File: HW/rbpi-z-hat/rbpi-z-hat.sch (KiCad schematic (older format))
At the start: 5 parts, among them Q1 DMG2302U

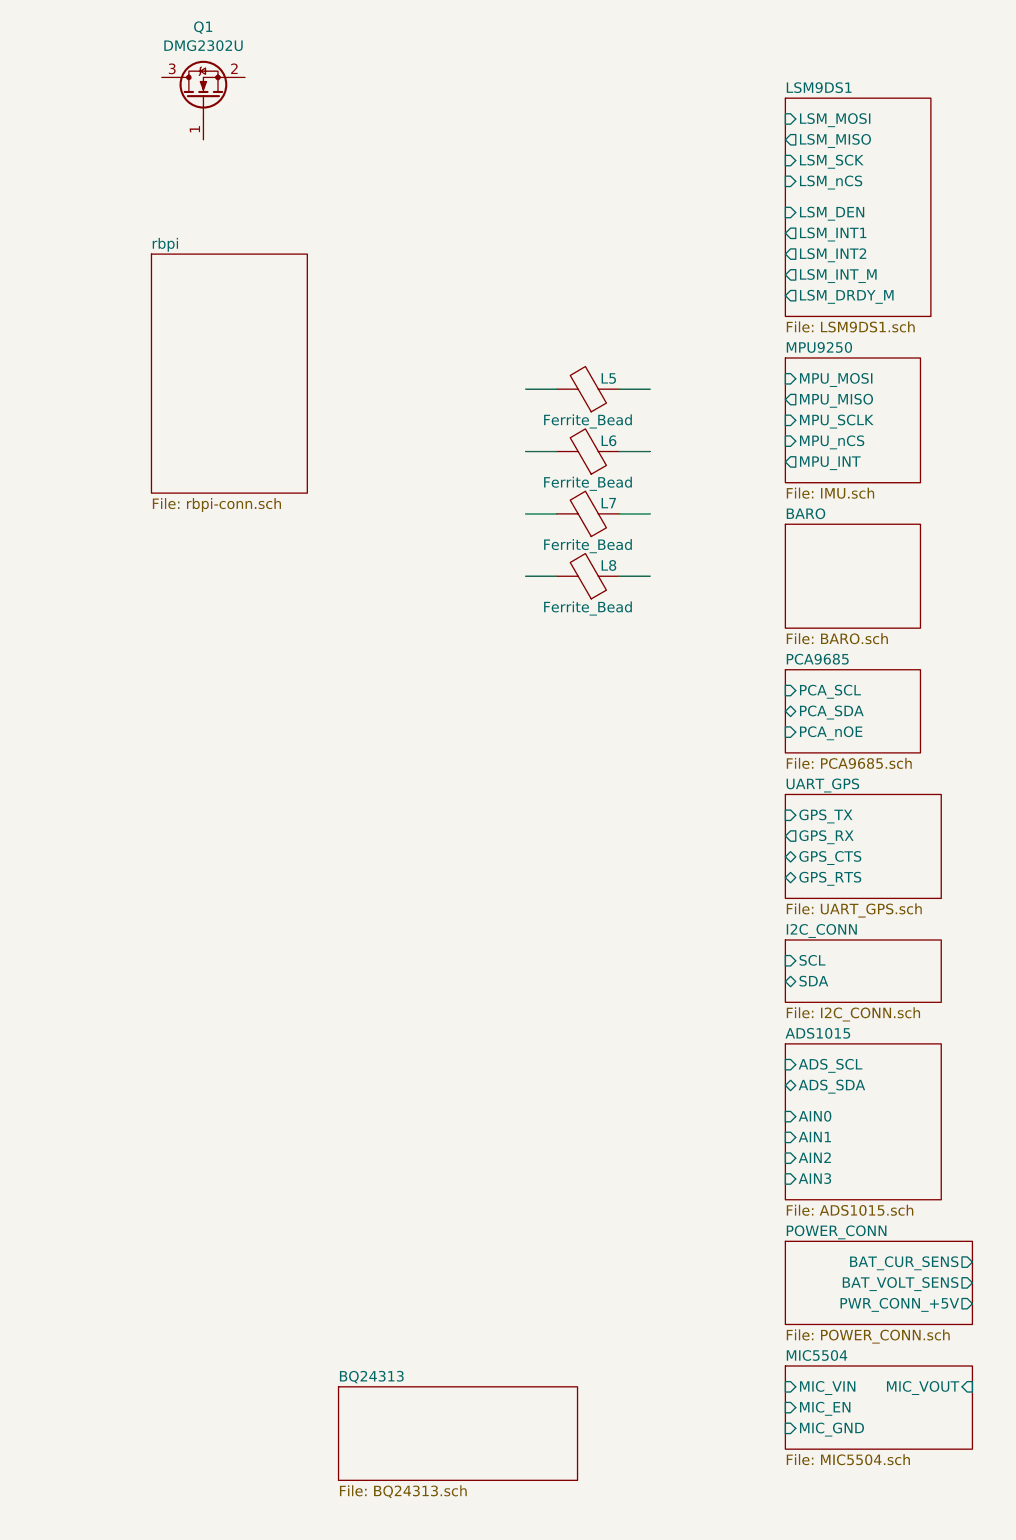
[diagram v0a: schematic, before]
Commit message: Commit...
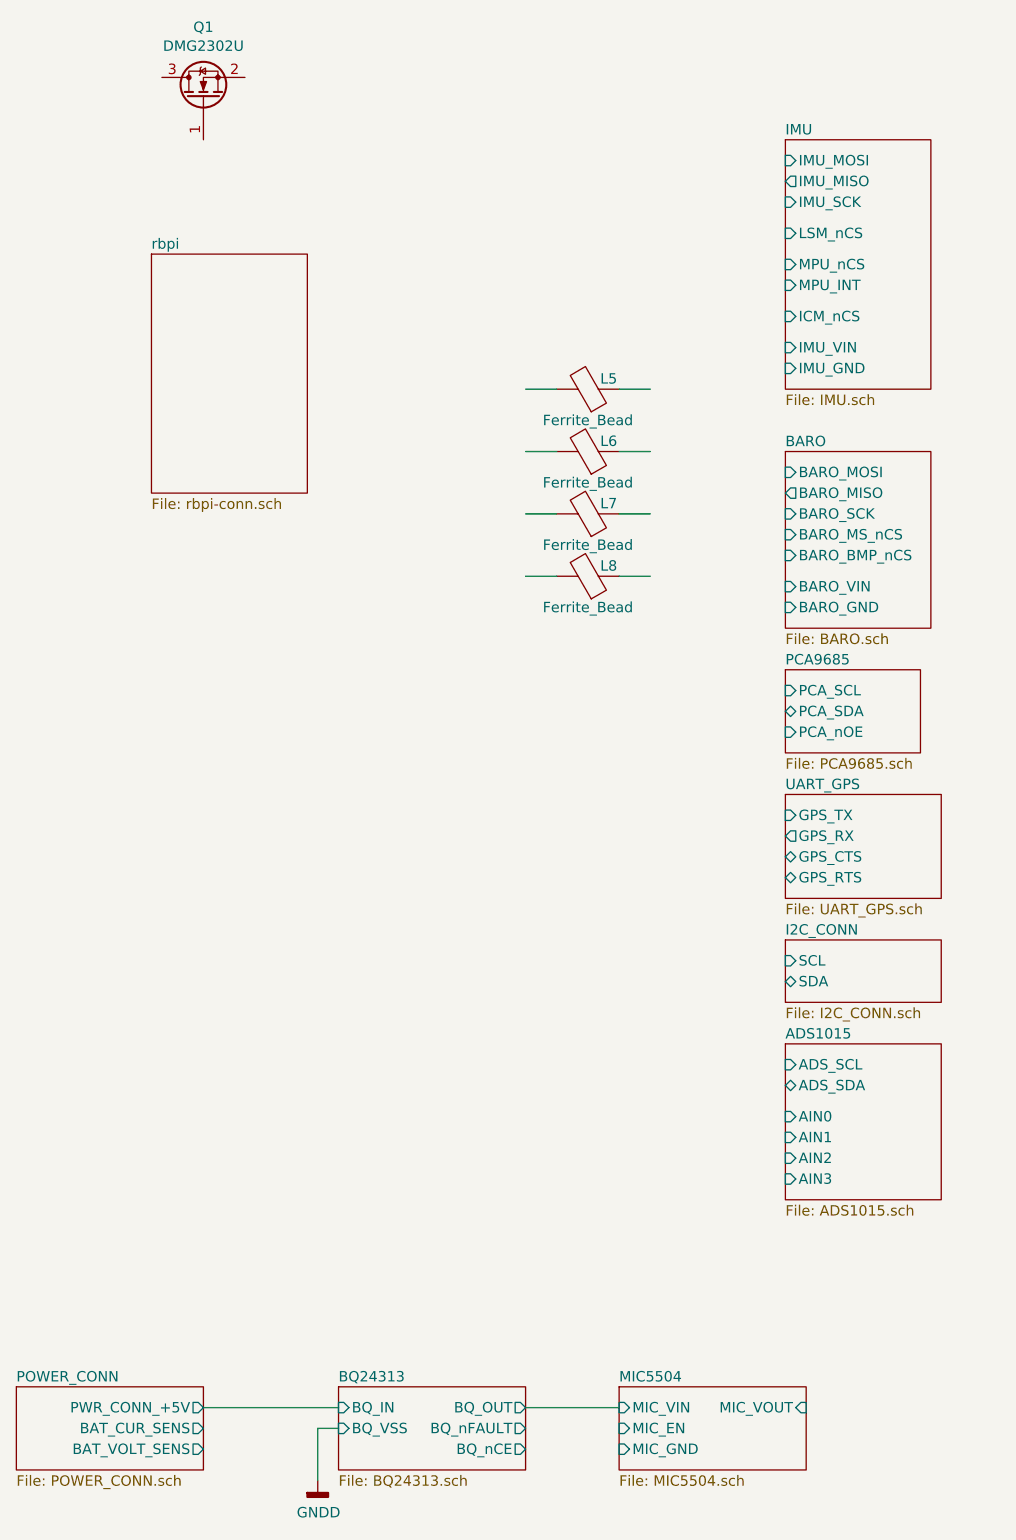
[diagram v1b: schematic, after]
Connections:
- net labels added: GNDD
- wire segments 8 -> 12
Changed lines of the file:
@@
 $Descr A4 8268 11693 portrait
 encoding utf-8
-Sheet 1 14
+Sheet 1 18
 Title "RasPi Zero NAV Hat"
 Date "2020-06-08"
@@
 $EndDescr
 $Sheet
-S 5200 2950 650  600
-U 5ED65008
-F0 "MPU9250" 50
-F1 "IMU.sch" 50
-F2 "MPU_MOSI" I L 5200 3050 50
-F3 "MPU_MISO" O L 5200 3150 50
-F4 "MPU_SCLK" I L 5200 3250 50
-F5 "MPU_nCS" I L 5200 3350 50
-F6 "MPU_INT" O L 5200 3450 50
-$EndSheet
-$Sheet
 S 5200 4450 650  400
 U 5ED666AD
@@
 	4550 4000 4400 4000
 $Sheet
-S 5200 1700 700  1050
-U 5F099163
-F0 "LSM9DS1" 50
-F1 "LSM9DS1.sch" 50
-F2 "LSM_SCK" I L 5200 2000 50
-F3 "LSM_INT1" O L 5200 2350 50
-F4 "LSM_INT2" O L 5200 2450 50
-F5 "LSM_DEN" I L 5200 2250 50
-F6 "LSM_nCS" I L 5200 2100 50
-F7 "LSM_INT_M" O L 5200 2550 50
-F8 "LSM_DRDY_M" O L 5200 2650 50
-F9 "LSM_MOSI" I L 5200 1800 50
-F10 "LSM_MISO" O L 5200 1900 50
-$EndSheet
-$Sheet
-S 5200 3750 650  500
+S 5200 3400 700  850
 U 5EF65A4D
 F0 "BARO" 50
 F1 "BARO.sch" 50
+F2 "BARO_VIN" I L 5200 4050 50
+F3 "BARO_MOSI" I L 5200 3500 50
+F4 "BARO_MISO" O L 5200 3600 50
+F5 "BARO_SCK" I L 5200 3700 50
+F6 "BARO_MS_nCS" I L 5200 3800 50
+F7 "BARO_BMP_nCS" I L 5200 3900 50
+F8 "BARO_GND" I L 5200 4150 50
 $EndSheet
 $Comp
@@
 $EndSheet
 $Sheet
-S 5200 7200 900  400
+S 1500 7900 900  400
 U 5EF28018
 F0 "POWER_CONN" 50
 F1 "POWER_CONN.sch" 50
-F2 "BAT_CUR_SENS" O R 6100 7300 50
-F3 "BAT_VOLT_SENS" O R 6100 7400 50
-F4 "PWR_CONN_+5V" O R 6100 7500 50
-$EndSheet
-$Sheet
-S 5200 7800 900  400
+F2 "BAT_CUR_SENS" O R 2400 8100 50
+F3 "BAT_VOLT_SENS" O R 2400 8200 50
+F4 "PWR_CONN_+5V" O R 2400 8000 50
+$EndSheet
+$Sheet
+S 4400 7900 900  400
 U 5EDADA57
 F0 "MIC5504" 50
 F1 "MIC5504.sch" 50
-F2 "MIC_EN" I L 5200 8000 50
-F3 "MIC_VIN" I L 5200 7900 50
-F4 "MIC_VOUT" I R 6100 7900 50
-F5 "MIC_GND" I L 5200 8100 50
-$EndSheet
-$Sheet
-S 3050 7900 1150 450
+F2 "MIC_EN" I L 4400 8100 50
+F3 "MIC_VIN" I L 4400 8000 50
+F4 "MIC_VOUT" I R 5300 8000 50
+F5 "MIC_GND" I L 4400 8200 50
+$EndSheet
+$Sheet
+S 3050 7900 900  400
 U 5EDDEA36
 F0 "BQ24313" 50
 F1 "BQ24313.sch" 50
+F2 "BQ_IN" I L 3050 8000 50
+F3 "BQ_VSS" I L 3050 8100 50
+F4 "BQ_nFAULT" O R 3950 8100 50
+F5 "BQ_OUT" O R 3950 8000 50
+F6 "BQ_nCE" O R 3950 8200 50
+$EndSheet
+Wire Wire Line
+	2400 8000 3050 8000
+$Comp
+L power:GNDD #PWR0106
+U 1 1 5EDEC12D
+P 2950 8350
+F 0 "#PWR0106" H 2950 8100 50  0001 C CNN
+F 1 "GNDD" H 2954 8195 50  0000 C CNN
+F 2 "" H 2950 8350 50  0001 C CNN
+F 3 "" H 2950 8350 50  0001 C CNN
+	1    2950 8350
+	1    0    0    -1
+$EndComp
+Wire Wire Line
+	3050 8100 2950 8100
+Wire Wire Line
+	2950 8100 2950 8350
+Wire Wire Line
+	3950 8000 4400 8000
+$Sheet
+S 5200 1900 700  1200
+U 5EE06F22
+F0 "IMU" 50
+F1 "IMU.sch" 50
+F2 "IMU_VIN" I L 5200 2900 50
+F3 "IMU_GND" I L 5200 3000 50
+F4 "IMU_MOSI" I L 5200 2000 50
+F5 "IMU_MISO" O L 5200 2100 50
+F6 "IMU_SCK" I L 5200 2200 50
+F7 "LSM_nCS" I L 5200 2350 50
+F8 "MPU_nCS" I L 5200 2500 50
+F9 "ICM_nCS" I L 5200 2750 50
+F10 "MPU_INT" I L 5200 2600 50
 $EndSheet
 $EndSCHEMATC
